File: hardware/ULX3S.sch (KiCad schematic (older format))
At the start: 2 parts

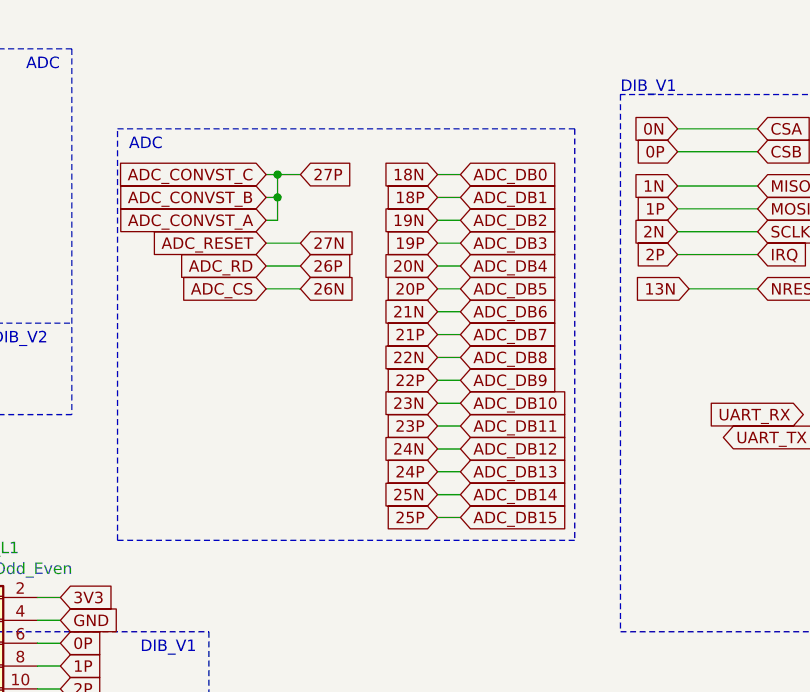
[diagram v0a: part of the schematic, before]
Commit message: Assigning footprints
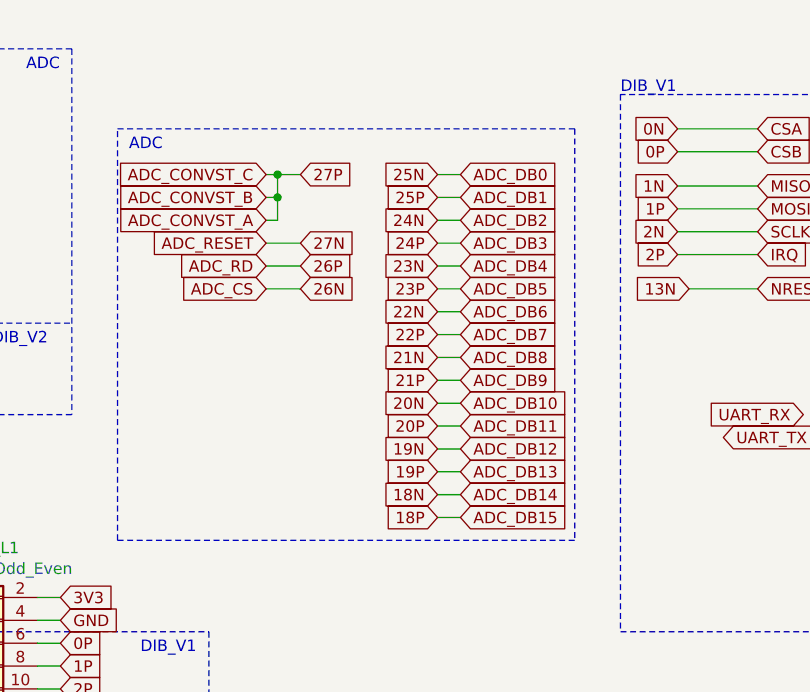
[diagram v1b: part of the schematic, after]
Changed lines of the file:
@@
 Text GLabel 4200 2200 0    50   Input ~ 0
 ADC_CS
-Text GLabel 4950 2600 0    50   Input ~ 0
+Text GLabel 4950 2400 0    50   Input ~ 0
 22P
-Text GLabel 4950 2500 0    50   Input ~ 0
+Text GLabel 4950 2300 0    50   Input ~ 0
 22N
 Wire Wire Line
@@
 Text GLabel 4350 2200 2    50   Input ~ 0
 26N
+Text GLabel 4950 1800 0    50   Input ~ 0
+25P
+Text GLabel 4950 1700 0    50   Input ~ 0
+25N
+Text GLabel 4950 2000 0    50   Input ~ 0
+24P
+Text GLabel 4950 1900 0    50   Input ~ 0
+24N
+Text GLabel 4950 2200 0    50   Input ~ 0
+23P
+Text GLabel 4950 2100 0    50   Input ~ 0
+23N
+Text GLabel 4950 2600 0    50   Input ~ 0
+21P
+Text GLabel 4950 2500 0    50   Input ~ 0
+21N
+Text GLabel 4950 2800 0    50   Input ~ 0
+20P
+Text GLabel 4950 2700 0    50   Input ~ 0
+20N
+Text GLabel 4950 3000 0    50   Input ~ 0
+19P
+Text GLabel 4950 2900 0    50   Input ~ 0
+19N
 Text GLabel 4950 3200 0    50   Input ~ 0
-25P
+18P
 Text GLabel 4950 3100 0    50   Input ~ 0
-25N
-Text GLabel 4950 3000 0    50   Input ~ 0
-24P
-Text GLabel 4950 2900 0    50   Input ~ 0
-24N
-Text GLabel 4950 2800 0    50   Input ~ 0
-23P
-Text GLabel 4950 2700 0    50   Input ~ 0
-23N
-Text GLabel 4950 2400 0    50   Input ~ 0
-21P
-Text GLabel 4950 2300 0    50   Input ~ 0
-21N
-Text GLabel 4950 2200 0    50   Input ~ 0
-20P
-Text GLabel 4950 2100 0    50   Input ~ 0
-20N
-Text GLabel 4950 2000 0    50   Input ~ 0
-19P
-Text GLabel 4950 1900 0    50   Input ~ 0
-19N
-Text GLabel 4950 1800 0    50   Input ~ 0
-18P
-Text GLabel 4950 1700 0    50   Input ~ 0
 18N
 Text Notes 1400 2450 0    50   ~ 0
